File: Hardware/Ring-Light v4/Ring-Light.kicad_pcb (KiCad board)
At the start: 4 copper layers, 115 x 142.5 mm, 179 parts, among them U1 NCR321PASX, U10 NCR321PASX, U11 NCR321PASX, U12 NCR321PASX, U13 NCR321PASX, U14 NCR321PASX, U15 NCR321PASX, U16 NCR321PASX, U17 NCR321PASX, U18 NCR321PASX, U19 NCR321PASX, U2 NCR321PASX, U20 NCR321PASX, U21 NCR321PASX, U22 NCR321PASX, U23 NCR321PASX, U24 NCR321PASX, U25 NCR321PASX, U26 NCR321PASX, U27 NCR321PASX, U28 NCR321PASX, U29 NCR321PASX, U3 NCR321PASX, U30 NCR321PASX, U31 NCR321PASX, U32 NCR321PASX, U33 PCA9685BS,118, U4 NCR321PASX, U5 NCR321PASX, U6 NCR321PASX, U7 NCR321PASX, U8 NCR321PASX, U9 NCR321PASX

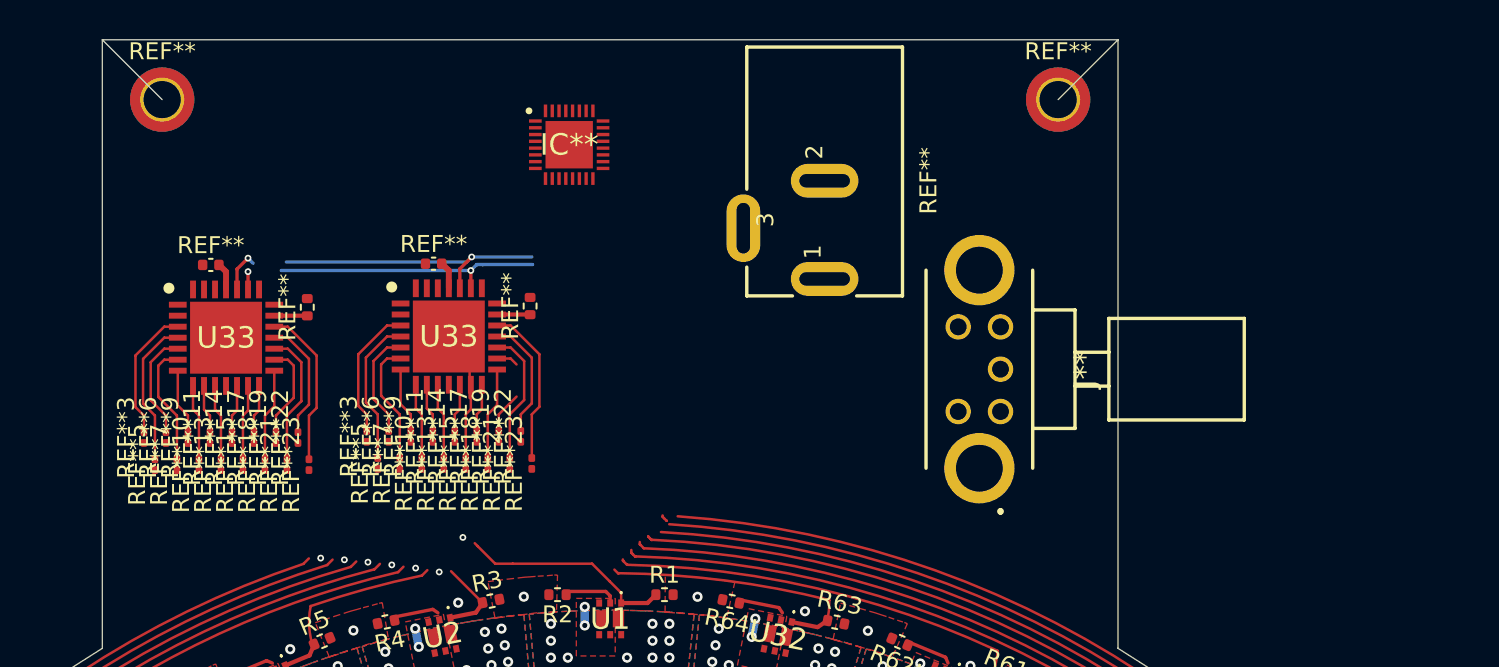
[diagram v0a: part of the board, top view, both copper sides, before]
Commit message: m
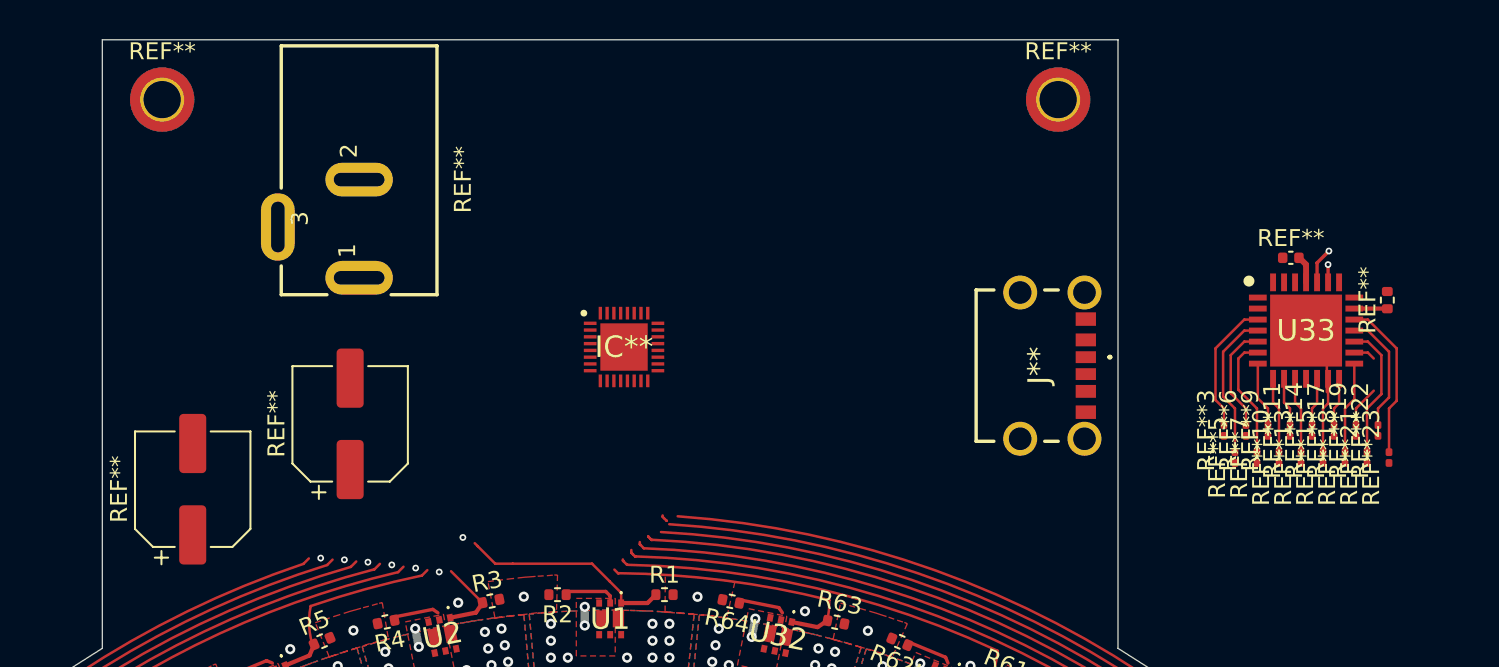
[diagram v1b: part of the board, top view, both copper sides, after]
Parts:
- removed the J** at (143.1, 37.0)
- removed the REF** at (102.1, 30.8)
- removed the REF** at (96.4, 28.3)
- removed the REF**10 at (95.7, 40.1)
- removed the REF**11 at (96.4, 38.5)
- removed the REF**13 at (97.0, 40.1)
- removed the REF**14 at (97.7, 38.5)
- removed the REF**15 at (98.3, 40.1)
- removed the REF**17 at (99.0, 38.5)
- removed the REF**18 at (99.6, 40.1)
- removed the REF**19 at (100.3, 38.5)
- removed the REF**21 at (100.9, 40.1)
- removed the REF**22 at (101.6, 38.5)
- removed the REF**23 at (102.2, 40.1)
- removed the REF**3 at (92.5, 38.5)
- removed the REF**5 at (93.1, 40.1)
- removed the REF**6 at (93.8, 38.5)
- removed the REF**7 at (94.4, 40.1)
- removed the REF**9 at (95.1, 38.5)
- removed the U33 at (97.3, 32.6)
- added J**: 2171750001, Library:2171750001, F.Cu at (145.1, 34.2)
- added REF**: CP_Elec_6.3x7.7, Capacitor_SMD:CP_Elec_6.3x7.7, F.Cu at (95.3, 41.5)
- added REF**: CP_Elec_6.3x7.7, Capacitor_SMD:CP_Elec_6.3x7.7, F.Cu at (104.6, 37.7)
- moved REF** 50.6 mm to (160.2, 27.9)
- moved REF**14 50.6 mm to (161.5, 38.1)
- moved REF**15 50.6 mm to (162.1, 39.7)
- moved REF**21 50.6 mm to (164.7, 39.7)
- moved REF**22 50.6 mm to (165.4, 38.1)
- moved REF**7 50.6 mm to (158.2, 39.7)
- moved REF**9 50.6 mm to (158.9, 38.1)
- moved U33 50.6 mm to (161.1, 32.2)
- moved REF** 50.6 mm to (165.9, 30.4)
- moved REF**11 50.6 mm to (160.2, 38.1)
- moved REF**13 50.6 mm to (160.8, 39.7)
- moved REF**18 50.6 mm to (163.4, 39.7)
- moved REF**19 50.6 mm to (164.1, 38.1)
- moved REF**5 50.6 mm to (156.9, 39.7)
- moved REF**6 50.6 mm to (157.6, 38.1)
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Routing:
- net SDA: track 19.3 -> 2.56 mm, vias 2 -> 1
- net SCL: track 17.1 -> 1.05 mm, vias 2 -> 1
- net Net-(U33-LED15): track 19.0 -> 9.52 mm
- net Net-(U33-LED1): track 17.6 -> 8.79 mm
- net Net-(U33-LED13): track 16.0 -> 8.01 mm
- net Net-(U33-LED0): track 15.9 -> 7.94 mm
- net Net-(U33-LED3): track 14.6 -> 7.28 mm
- net Net-(U33-LED14): track 14.4 -> 7.19 mm
- net Net-(U33-LED2): track 12.9 -> 6.43 mm
- net Net-(U33-LED12): track 11.3 -> 5.66 mm
- net Net-(U33-LED11): track 10.9 -> 5.46 mm
- net Net-(U33-LED7): track 8.99 -> 4.49 mm
- net Net-(U33-LED5): track 8.95 -> 4.47 mm
- net Net-(U33-LED9): track 8.91 -> 4.45 mm
- net Net-(U33-LED4): track 7.76 -> 3.88 mm
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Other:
- outline, holes or cut-outs redrawn

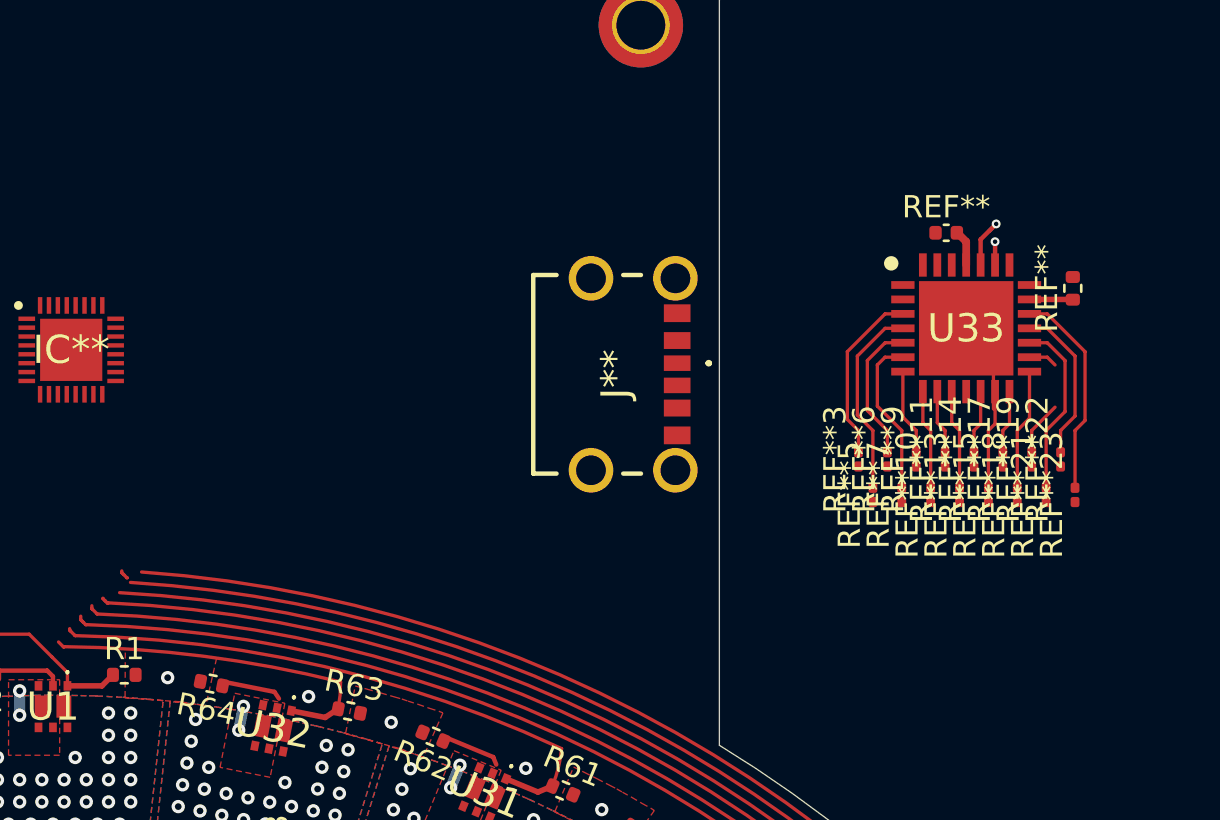
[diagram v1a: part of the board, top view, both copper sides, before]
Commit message: d
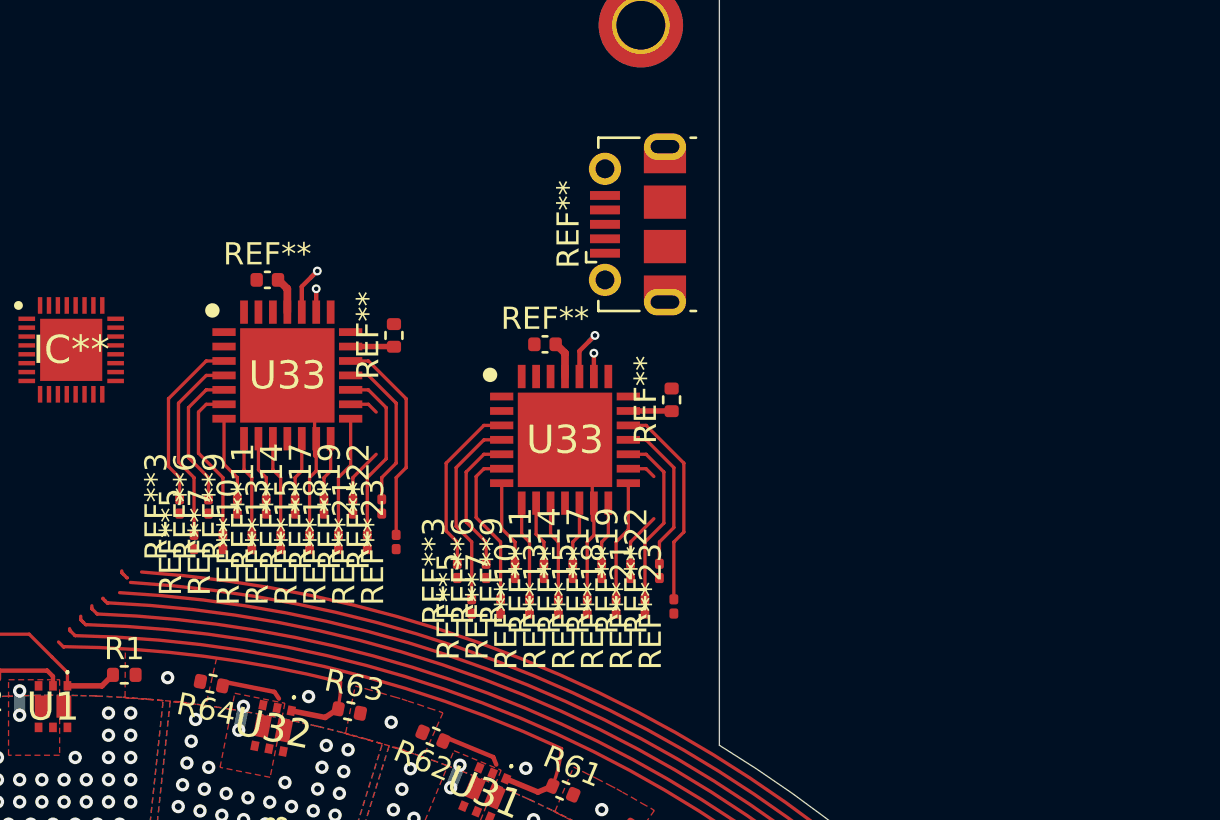
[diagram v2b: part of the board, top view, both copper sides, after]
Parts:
- removed J**: 2171750001, Library:2171750001
- added REF**: R_0402_1005Metric, Resistor_SMD:R_0402_1005Metric, F.Cu at (135.3, 32.5)
- added REF**: USB_Micro-B_Molex-105017-0001, Connector_USB:USB_Micro-B_Molex-105017-0001, F.Cu at (146.3, 27.5)
- added REF**: C_0402_1005Metric, Capacitor_SMD:C_0402_1005Metric, F.Cu at (129.7, 30.0)
- added REF**10: R_0201_0603Metric, Resistor_SMD:R_0201_0603Metric, F.Cu at (128.9, 41.8)
- added REF**11: R_0201_0603Metric, Resistor_SMD:R_0201_0603Metric, F.Cu at (129.6, 40.2)
- added REF**13: R_0201_0603Metric, Resistor_SMD:R_0201_0603Metric, F.Cu at (130.2, 41.8)
- added REF**14: R_0201_0603Metric, Resistor_SMD:R_0201_0603Metric, F.Cu at (130.9, 40.2)
- added REF**15: R_0201_0603Metric, Resistor_SMD:R_0201_0603Metric, F.Cu at (131.6, 41.8)
- added REF**17: R_0201_0603Metric, Resistor_SMD:R_0201_0603Metric, F.Cu at (132.2, 40.2)
- added REF**18: R_0201_0603Metric, Resistor_SMD:R_0201_0603Metric, F.Cu at (132.8, 41.8)
- added REF**19: R_0201_0603Metric, Resistor_SMD:R_0201_0603Metric, F.Cu at (133.5, 40.2)
- added REF**21: R_0201_0603Metric, Resistor_SMD:R_0201_0603Metric, F.Cu at (134.2, 41.8)
- added REF**22: R_0201_0603Metric, Resistor_SMD:R_0201_0603Metric, F.Cu at (134.8, 40.2)
- added REF**23: R_0201_0603Metric, Resistor_SMD:R_0201_0603Metric, F.Cu at (135.4, 41.8)
- added REF**3: R_0201_0603Metric, Resistor_SMD:R_0201_0603Metric, F.Cu at (125.7, 40.2)
- added REF**5: R_0201_0603Metric, Resistor_SMD:R_0201_0603Metric, F.Cu at (126.3, 41.8)
- added REF**6: R_0201_0603Metric, Resistor_SMD:R_0201_0603Metric, F.Cu at (127.0, 40.2)
- added REF**7: R_0201_0603Metric, Resistor_SMD:R_0201_0603Metric, F.Cu at (127.7, 41.8)
- added REF**9: R_0201_0603Metric, Resistor_SMD:R_0201_0603Metric, F.Cu at (128.3, 40.2)
- added U33: PCA9685BS,118, Library:QFN65P600X600X100-29N-D, F.Cu at (130.6, 34.3)
- moved REF**10 18.7 mm to (141.4, 44.7)
- moved REF**11 18.7 mm to (142.1, 43.1)
- moved REF**13 18.7 mm to (142.8, 44.7)
- moved REF**14 18.7 mm to (143.4, 43.1)
- moved REF**15 18.7 mm to (144.1, 44.7)
- moved REF**17 18.7 mm to (144.7, 43.1)
- moved REF**18 18.7 mm to (145.3, 44.7)
- moved REF**19 18.7 mm to (146.0, 43.1)
- moved REF**21 18.7 mm to (146.7, 44.7)
- moved REF**22 18.7 mm to (147.3, 43.1)
- moved REF**23 18.7 mm to (147.9, 44.7)
- moved REF**3 18.7 mm to (138.2, 43.1)
- moved REF**5 18.7 mm to (138.8, 44.7)
- moved REF**6 18.7 mm to (139.5, 43.1)
- moved REF**7 18.7 mm to (140.2, 44.7)
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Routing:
- net Net-(U33-LED15): track 9.52 -> 19.0 mm
- net Net-(U33-LED1): track 8.79 -> 17.6 mm
- net Net-(U33-LED13): track 8.01 -> 16.0 mm
- net Net-(U33-LED0): track 7.94 -> 15.9 mm
- net Net-(U33-LED3): track 7.28 -> 14.6 mm
- net Net-(U33-LED14): track 7.19 -> 14.4 mm
- net Net-(U33-LED2): track 6.43 -> 12.9 mm
- net Net-(U33-LED12): track 5.66 -> 11.3 mm
- net Net-(U33-LED11): track 5.46 -> 10.9 mm
- net Net-(U33-LED7): track 4.49 -> 8.99 mm
- net Net-(U33-LED5): track 4.47 -> 8.95 mm
- net Net-(U33-LED9): track 4.45 -> 8.91 mm
- net Net-(U33-LED4): track 3.88 -> 7.76 mm
- net Net-(U33-LED6): track 2.87 -> 5.75 mm
- net Net-(U33-LED10): track 2.85 -> 5.71 mm
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
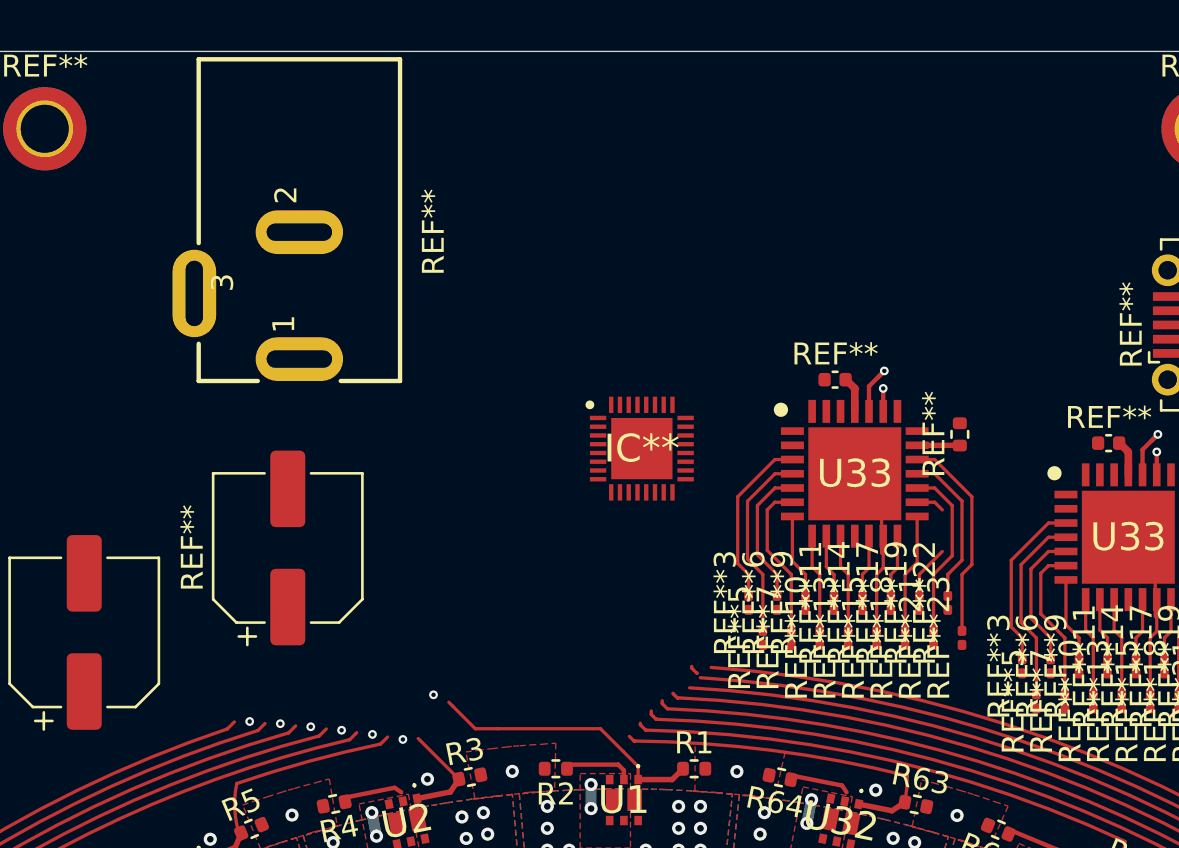
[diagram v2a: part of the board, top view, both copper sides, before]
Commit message: m
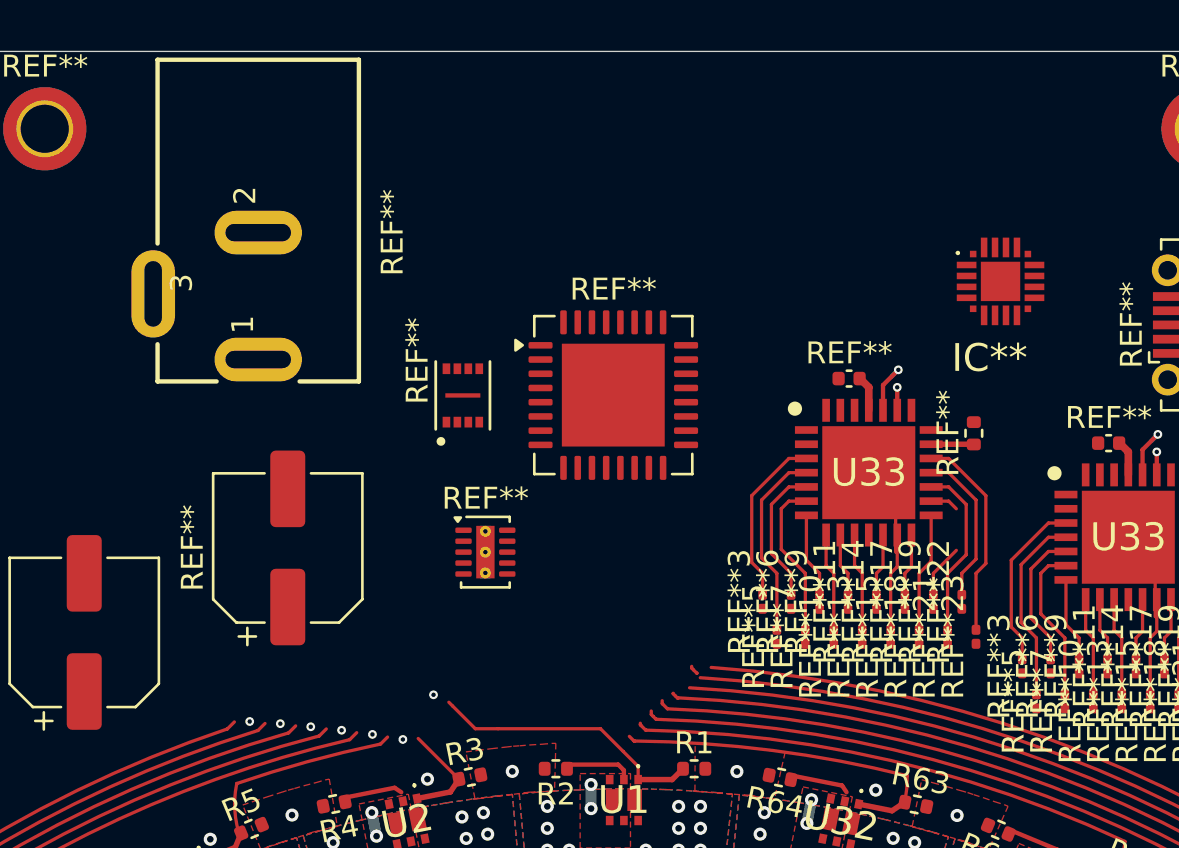
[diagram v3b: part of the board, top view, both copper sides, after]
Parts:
- removed the IC** at (120.8, 33.1)
- added IC**: CP2102NA02GQFN20, Library:CP2102NA02GQFN20, F.Cu at (137.2, 25.5)
- added REF**: PSON50P300X200X60-9N, Library:PSON50P300X200X60-9N, F.Cu at (112.6, 30.7)
- added REF**: QFN-32-1EP_7x7mm_P0.65mm_EP4.7x4.7mm, Package_DFN_QFN:QFN-32-1EP_7x7mm_P0.65mm_EP4.7x4.7mm, F.Cu at (119.5, 30.7)
- added REF**: WSON-10-1EP_2x3mm_P0.5mm_EP0.84x2.4mm_ThermalVias, Package_SON:WSON-10-1EP_2x3mm_P0.5mm_EP0.84x2.4mm_ThermalVias, F.Cu at (113.7, 37.9)
- moved REF** 1.88 mm to (103.3, 23.3)
- moved REF**11 0.64 mm to (130.2, 40.1)
- moved REF**17 0.64 mm to (132.8, 40.1)
- moved REF** 0.64 mm to (136.0, 32.5)
- moved REF**10 0.64 mm to (129.6, 41.8)
- moved REF**18 0.64 mm to (133.5, 41.8)
- moved REF**23 0.64 mm to (136.1, 41.8)
- moved REF**3 0.64 mm to (126.3, 40.1)
- moved REF**6 0.64 mm to (127.6, 40.1)
- moved REF**5 0.64 mm to (127.0, 41.8)
- moved REF**14 0.64 mm to (131.5, 40.1)
- moved REF**19 0.64 mm to (134.1, 40.1)
- moved REF**22 0.64 mm to (135.4, 40.1)
- moved REF**9 0.64 mm to (128.9, 40.1)
- moved REF** 0.64 mm to (130.3, 29.9)
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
